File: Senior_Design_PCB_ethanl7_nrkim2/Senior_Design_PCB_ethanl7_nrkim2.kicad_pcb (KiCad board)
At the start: 2 copper layers, 127 x 127 mm, 86 parts, among them J1 Piezo, J10 M6, J2 9V supply battery or bench, J3 Conn_02x03_Odd_Even, J4 Conn_ARM_JTAG_SWD_10, J5 M1, J6 M2, J7 M3, J8 M4, J9 M5, SW1 SW_Push, U1 uA7805, U2 LM386, U3 L298N, U4 L298N, U5 L298N, U6 STM32H7B0RBTx, U7 LM2937xT

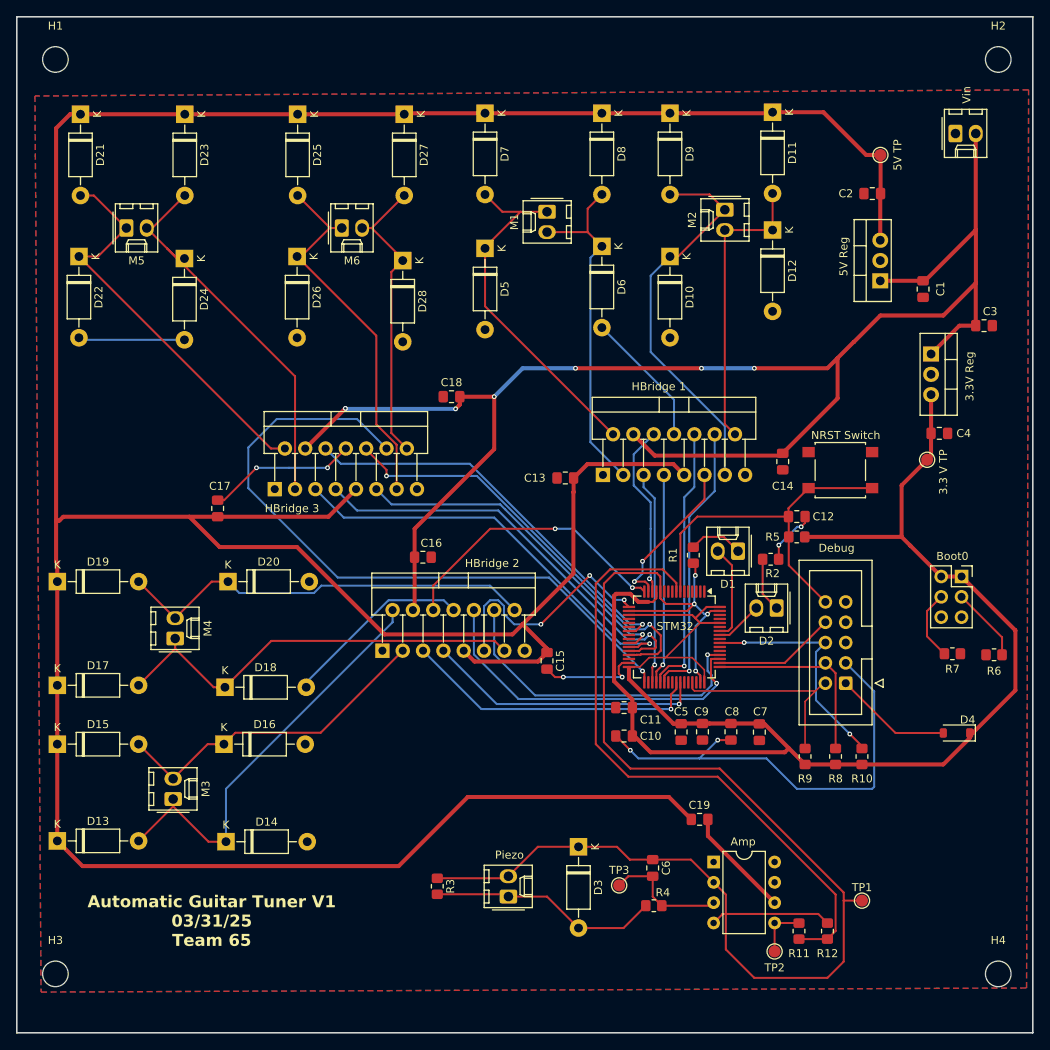
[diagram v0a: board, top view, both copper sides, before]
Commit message: V1.1 pcb
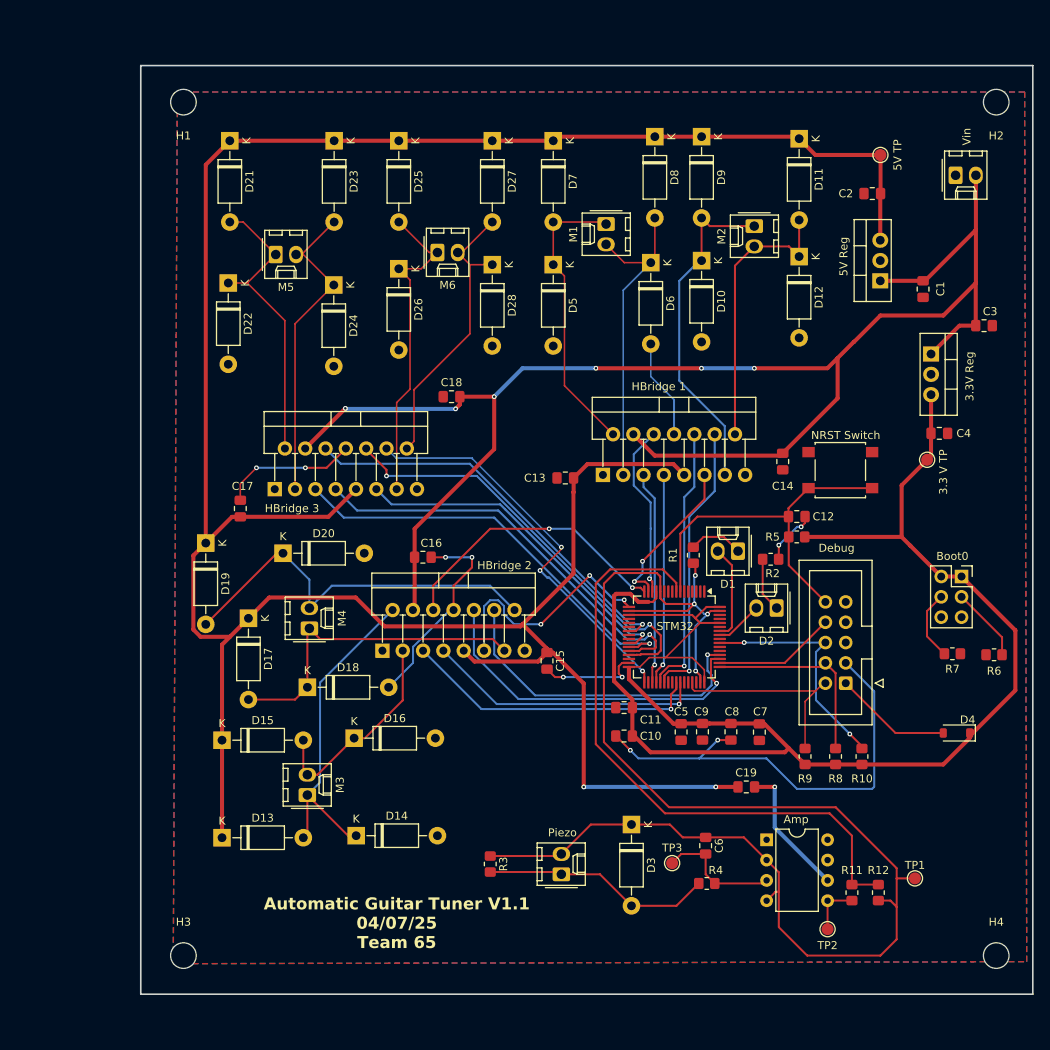
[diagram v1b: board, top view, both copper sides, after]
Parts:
- moved D17 25.3 mm to (109.0, 100.1), turned to -90 degrees
- moved D15 20.6 mm to (105.7, 115.3)
- moved D13 20.6 mm to (105.7, 127.5)
- moved D19 19.2 mm to (103.6, 90.7), turned to -90 degrees
- moved D22 19.0 mm to (106.4, 58.2)
- moved D21 19.0 mm to (106.6, 40.4)
- moved D23 19.0 mm to (119.7, 40.4)
- moved D24 19.0 mm to (119.6, 58.4)
- moved J9 19.0 mm to (112.4, 54.6)
- moved H1 16.9 mm to (100.8, 35.6), turned to 180 degrees
- moved J8 16.8 mm to (116.6, 101.3)
- moved J7 16.8 mm to (116.3, 122.2)
- moved D16 16.3 mm to (122.2, 115.1)
- moved D14 16.3 mm to (122.4, 127.3)
- moved H3 16.2 mm to (100.8, 142.2)
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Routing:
- net +5V: track 430.9 -> 339.1 mm, vias 0 -> 2
- net /M6N: track 85.6 -> 50.6 mm, vias 1 -> 3
- net GND: track 339.5 -> 317.1 mm, vias 12 -> 14
- net Net-(D15-A): track 41.4 -> 26.5 mm
- net Net-(D21-A): track 50.5 -> 37.5 mm
- net Net-(D17-A): track 53.8 -> 41.0 mm
- net Net-(D13-A): track 53.0 -> 41.3 mm
- net Net-(D23-A): track 49.5 -> 40.3 mm
- net Net-(D5-K): track 44.9 -> 36.3 mm
- net Net-(D10-K): track 49.1 -> 42.8 mm
- net Net-(D25-A): track 47.0 -> 40.9 mm
- net +9V: track 204.3 -> 199.0 mm
- net Net-(D6-K): track 43.9 -> 40.3 mm
- net Net-(D19-A): track 53.0 -> 49.6 mm
- net Net-(U2-V+): track 13.9 -> 16.9 mm, vias 0 -> 1
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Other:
- board size 127 x 127 mm -> 111.5 x 116.1 mm
- board text added: "Automatic Guitar Tuner V1.1 04/07/25 Team 65"
- board text removed: "Automatic Guitar Tuner V1 03/31/25 Team 65"
